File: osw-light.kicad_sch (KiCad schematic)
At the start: 53 parts, among them J1 Conn_01x02, J2 USB_C_Receptacle_USB2.0, Q1 2N7002, SW1 SW_Push, SW2 SW_Push, SW4 SW_Push, SW5 SW_Push, U1 DS3231MZ, U10 XC6209, U11 MCP73831T-2ACI_OT, U13 XC6209, U2 BMA400, U4 GC9A01_IPS_display, U6 CH340E, U7 ttgo-32-micro, U9 TPS2115A

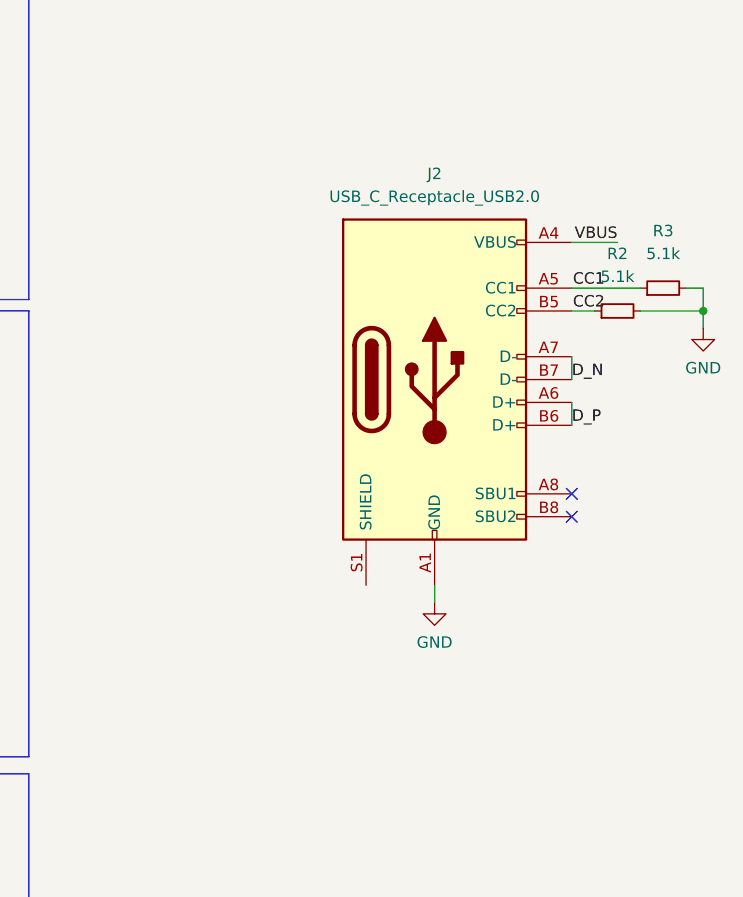
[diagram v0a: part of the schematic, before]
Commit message: fixed some footprints and other stuff
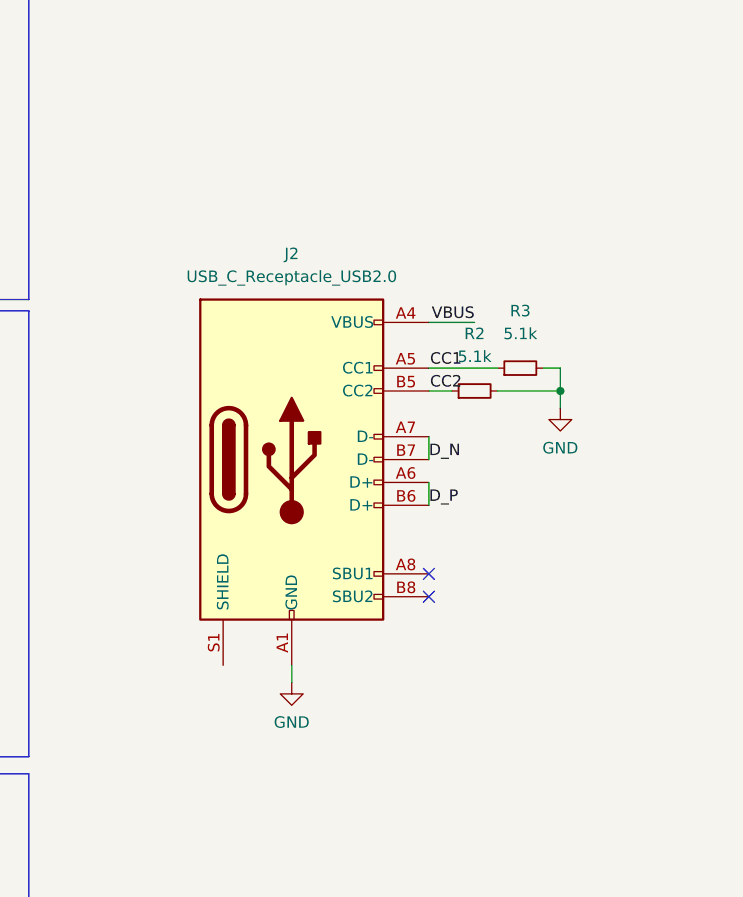
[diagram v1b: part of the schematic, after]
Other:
- moved on the sheet: J2, R2, R3
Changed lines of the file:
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@@
   (junction (at 33.02 156.21) (diameter 0) (color 0 0 0 0)
   )
-  (junction (at 356.87 63.5) (diameter 0) (color 0 0 0 0)
+  (junction (at 340.995 72.39) (diameter 0) (color 0 0 0 0)
   )
   (junction (at 159.385 172.72) (diameter 0) (color 0 0 0 0)
@@
   (no_connect (at 217.17 86.36))
   (no_connect (at 29.21 86.36))
-  (no_connect (at 342.265 83.82))
-  (no_connect (at 342.265 86.36))
+  (no_connect (at 326.39 92.71))
+  (no_connect (at 326.39 95.25))
   (polyline (pts (xy 208.28 114.935) (xy 281.94 114.935))
     (stroke (width 0) (type default) (color 0 0 0 0))
   )
-  (wire (pts (xy 342.265 60.96) (xy 349.885 60.96))
+  (wire (pts (xy 326.39 69.85) (xy 334.01 69.85))
     (stroke (width 0) (type default) (color 0 0 0 0))
   )
@@
     (stroke (width 0) (type default) (color 0 0 0 0))
   )
-  (wire (pts (xy 354.965 60.96) (xy 356.87 60.96))
+  (wire (pts (xy 339.09 69.85) (xy 340.995 69.85))
     (stroke (width 0) (type default) (color 0 0 0 0))
   )
@@
     (stroke (width 0) (type default) (color 0 0 0 0))
   )
-  (wire (pts (xy 356.87 63.5) (xy 356.87 65.405))
+  (wire (pts (xy 340.995 72.39) (xy 340.995 74.295))
     (stroke (width 0) (type default) (color 0 0 0 0))
   )
@@
     (stroke (width 0) (type default) (color 0 0 0 0))
   )
-  (wire (pts (xy 342.265 73.66) (xy 342.265 76.2))
+  (wire (pts (xy 326.39 82.55) (xy 326.39 85.09))
     (stroke (width 0) (type default) (color 0 0 0 0))
   )
@@
     (stroke (width 0) (type default) (color 0 0 0 0))
   )
-  (wire (pts (xy 342.265 68.58) (xy 342.265 71.12))
+  (wire (pts (xy 326.39 77.47) (xy 326.39 80.01))
     (stroke (width 0) (type default) (color 0 0 0 0))
   )
@@
     (stroke (width 0) (type default) (color 0 0 0 0))
   )
-  (wire (pts (xy 356.87 63.5) (xy 349.885 63.5))
+  (wire (pts (xy 340.995 72.39) (xy 334.01 72.39))
     (stroke (width 0) (type default) (color 0 0 0 0))
   )
@@
     (stroke (width 0) (type default) (color 0 0 0 0))
   )
-  (wire (pts (xy 342.265 55.88) (xy 347.345 55.88))
+  (wire (pts (xy 326.39 64.77) (xy 331.47 64.77))
     (stroke (width 0) (type default) (color 0 0 0 0))
   )
@@
     (stroke (width 0) (type default) (color 0 0 0 0))
   )
-  (wire (pts (xy 327.025 93.98) (xy 327.025 95.885))
+  (wire (pts (xy 311.15 102.87) (xy 311.15 104.775))
     (stroke (width 0) (type default) (color 0 0 0 0))
   )
@@
     (stroke (width 0) (type default) (color 0 0 0 0))
   )
-  (wire (pts (xy 342.265 63.5) (xy 344.805 63.5))
+  (wire (pts (xy 326.39 72.39) (xy 328.93 72.39))
     (stroke (width 0) (type default) (color 0 0 0 0))
   )
@@
     (stroke (width 0) (type default) (color 0 0 0 0))
   )
-  (wire (pts (xy 356.87 60.96) (xy 356.87 63.5))
+  (wire (pts (xy 340.995 69.85) (xy 340.995 72.39))
     (stroke (width 0) (type default) (color 0 0 0 0))
   )
@@
     (effects (font (size 1.27 1.27)) (justify left bottom))
   )
-  (label "D_N" (at 342.265 71.12 0)
-    (effects (font (size 1.27 1.27)) (justify left bottom))
-  )
-  (label "VBUS" (at 347.345 55.88 180)
+  (label "D_N" (at 326.39 80.01 0)
+    (effects (font (size 1.27 1.27)) (justify left bottom))
+  )
+  (label "VBUS" (at 331.47 64.77 180)
     (effects (font (size 1.27 1.27)) (justify right bottom))
   )
@@
     (effects (font (size 1.27 1.27)) (justify left bottom))
   )
-  (label "CC2" (at 342.392 63.5 0)
+  (label "CC2" (at 326.517 72.39 0)
     (effects (font (size 1.27 1.27)) (justify left bottom))
   )
@@
     (effects (font (size 1.27 1.27)) (justify left bottom))
   )
-  (label "D_P" (at 342.265 76.2 0)
+  (label "D_P" (at 326.39 85.09 0)
     (effects (font (size 1.27 1.27)) (justify left bottom))
   )
@@
     (effects (font (size 1.27 1.27)) (justify right bottom))
   )
-  (label "CC1" (at 342.392 60.96 0)
+  (label "CC1" (at 326.517 69.85 0)
     (effects (font (size 1.27 1.27)) (justify left bottom))
   )
@@
     (pin "1")
   )
-  (symbol (lib_id "Connector:USB_C_Receptacle_USB2.0") (at 327.025 71.12 0) (unit 1)
+  (symbol (lib_id "Connector:USB_C_Receptacle_USB2.0") (at 311.15 80.01 0) (unit 1)
     (in_bom yes) (on_board yes) (fields_autoplaced)
-    (property "Reference" "J2" (id 0) (at 327.025 48.26 0))
-    (property "Value" "USB_C_Receptacle_USB2.0" (id 1) (at 327.025 50.8 0))
-    (property "Footprint" "sat1l:GCT_USB4105-GF-A" (id 2) (at 330.835 71.12 0)
-      (effects (font (size 1.27 1.27)) hide)
-    )
-    (property "Datasheet" "https://www.usb.org/sites/default/files/documents/usb_type-c.zip" (id 3) (at 330.835 71.12 0)
+    (property "Reference" "J2" (id 0) (at 311.15 57.15 0))
+    (property "Value" "USB_C_Receptacle_USB2.0" (id 1) (at 311.15 59.69 0))
+    (property "Footprint" "sat1l:GCT_USB4105-GF-A" (id 2) (at 314.96 80.01 0)
+      (effects (font (size 1.27 1.27)) hide)
+    )
+    (property "Datasheet" "https://www.usb.org/sites/default/files/documents/usb_type-c.zip" (id 3) (at 314.96 80.01 0)
       (effects (font (size 1.27 1.27)) hide)
     )
@@
     (pin "S1")
   )
-  (symbol (lib_id "Device:R_Small") (at 347.345 63.5 90) (unit 1)
+  (symbol (lib_id "Device:R_Small") (at 331.47 72.39 90) (unit 1)
     (in_bom yes) (on_board yes) (fields_autoplaced)
-    (property "Reference" "R2" (id 0) (at 347.345 57.15 90))
-    (property "Value" "5.1k" (id 1) (at 347.345 59.69 90))
-    (property "Footprint" "Resistor_SMD:R_0603_1608Metric" (id 2) (at 347.345 63.5 0)
-      (effects (font (size 1.27 1.27)) hide)
-    )
-    (property "Datasheet" "~" (id 3) (at 347.345 63.5 0)
-      (effects (font (size 1.27 1.27)) hide)
-    )
-    (pin "1")
-    (pin "2")
-  )
-  (symbol (lib_id "Device:R_Small") (at 352.425 60.96 90) (unit 1)
+    (property "Reference" "R2" (id 0) (at 331.47 66.04 90))
+    (property "Value" "5.1k" (id 1) (at 331.47 68.58 90))
+    (property "Footprint" "Resistor_SMD:R_0603_1608Metric" (id 2) (at 331.47 72.39 0)
+      (effects (font (size 1.27 1.27)) hide)
+    )
+    (property "Datasheet" "~" (id 3) (at 331.47 72.39 0)
+      (effects (font (size 1.27 1.27)) hide)
+    )
+    (pin "1")
+    (pin "2")
+  )
+  (symbol (lib_id "Device:R_Small") (at 336.55 69.85 90) (unit 1)
     (in_bom yes) (on_board yes) (fields_autoplaced)
-    (property "Reference" "R3" (id 0) (at 352.425 54.61 90))
-    (property "Value" "5.1k" (id 1) (at 352.425 57.15 90))
-    (property "Footprint" "Resistor_SMD:R_0603_1608Metric" (id 2) (at 352.425 60.96 0)
-      (effects (font (size 1.27 1.27)) hide)
-    )
-    (property "Datasheet" "~" (id 3) (at 352.425 60.96 0)
-      (effects (font (size 1.27 1.27)) hide)
-    )
-    (pin "1")
-    (pin "2")
-  )
-  (symbol (lib_id "power:GND") (at 327.025 95.885 0) (unit 1)
+    (property "Reference" "R3" (id 0) (at 336.55 63.5 90))
+    (property "Value" "5.1k" (id 1) (at 336.55 66.04 90))
+    (property "Footprint" "Resistor_SMD:R_0603_1608Metric" (id 2) (at 336.55 69.85 0)
+      (effects (font (size 1.27 1.27)) hide)
+    )
+    (property "Datasheet" "~" (id 3) (at 336.55 69.85 0)
+      (effects (font (size 1.27 1.27)) hide)
+    )
+    (pin "1")
+    (pin "2")
+  )
+  (symbol (lib_id "power:GND") (at 311.15 104.775 0) (unit 1)
     (in_bom yes) (on_board yes) (fields_autoplaced)
-    (property "Reference" "#PWR01" (id 0) (at 327.025 102.235 0)
-      (effects (font (size 1.27 1.27)) hide)
-    )
-    (property "Value" "GND" (id 1) (at 327.025 100.33 0))
-    (property "Footprint" "" (id 2) (at 327.025 95.885 0)
-      (effects (font (size 1.27 1.27)) hide)
-    )
-    (property "Datasheet" "" (id 3) (at 327.025 95.885 0)
-      (effects (font (size 1.27 1.27)) hide)
-    )
-    (pin "1")
-  )
-  (symbol (lib_id "power:GND") (at 356.87 65.405 0) (unit 1)
+    (property "Reference" "#PWR01" (id 0) (at 311.15 111.125 0)
+      (effects (font (size 1.27 1.27)) hide)
+    )
+    (property "Value" "GND" (id 1) (at 311.15 109.22 0))
+    (property "Footprint" "" (id 2) (at 311.15 104.775 0)
+      (effects (font (size 1.27 1.27)) hide)
+    )
+    (property "Datasheet" "" (id 3) (at 311.15 104.775 0)
+      (effects (font (size 1.27 1.27)) hide)
+    )
+    (pin "1")
+  )
+  (symbol (lib_id "power:GND") (at 340.995 74.295 0) (unit 1)
     (in_bom yes) (on_board yes) (fields_autoplaced)
-    (property "Reference" "#PWR02" (id 0) (at 356.87 71.755 0)
-      (effects (font (size 1.27 1.27)) hide)
-    )
-    (property "Value" "GND" (id 1) (at 356.87 69.85 0))
-    (property "Footprint" "" (id 2) (at 356.87 65.405 0)
-      (effects (font (size 1.27 1.27)) hide)
-    )
-    (property "Datasheet" "" (id 3) (at 356.87 65.405 0)
-      (effects (font (size 1.27 1.27)) hide)
-    )
+    (property "Reference" "#PWR02" (id 0) (at 340.995 80.645 0)
+      (effects (font (size 1.27 1.27)) hide)
+    )
+    (property "Value" "GND" (id 1) (at 340.995 78.74 0))
+    (property "Footprint" "" (id 2) (at 340.995 74.295 0)
+      (effects (font (size 1.27 1.27)) hide)
+    )
+    (property "Datasheet" "" (id 3) (at 340.995 74.295 0)
+      (effects (font (size 1.27 1.27)) hide)
+    )
